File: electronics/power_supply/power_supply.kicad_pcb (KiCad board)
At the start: 2 copper layers, 7 parts, among them J1 INPUT, T1 RSPRO_121-3824, U1 NCP3334

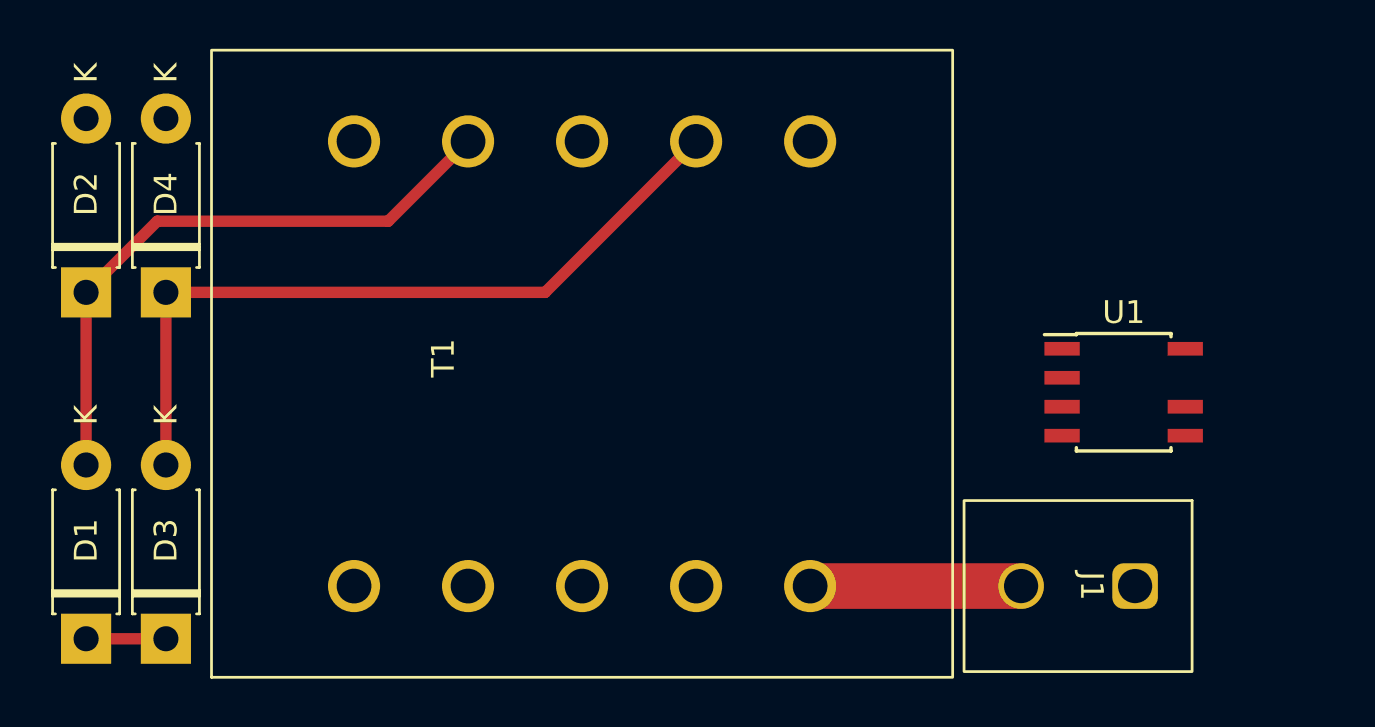
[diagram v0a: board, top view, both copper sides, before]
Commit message: power supply done, to check
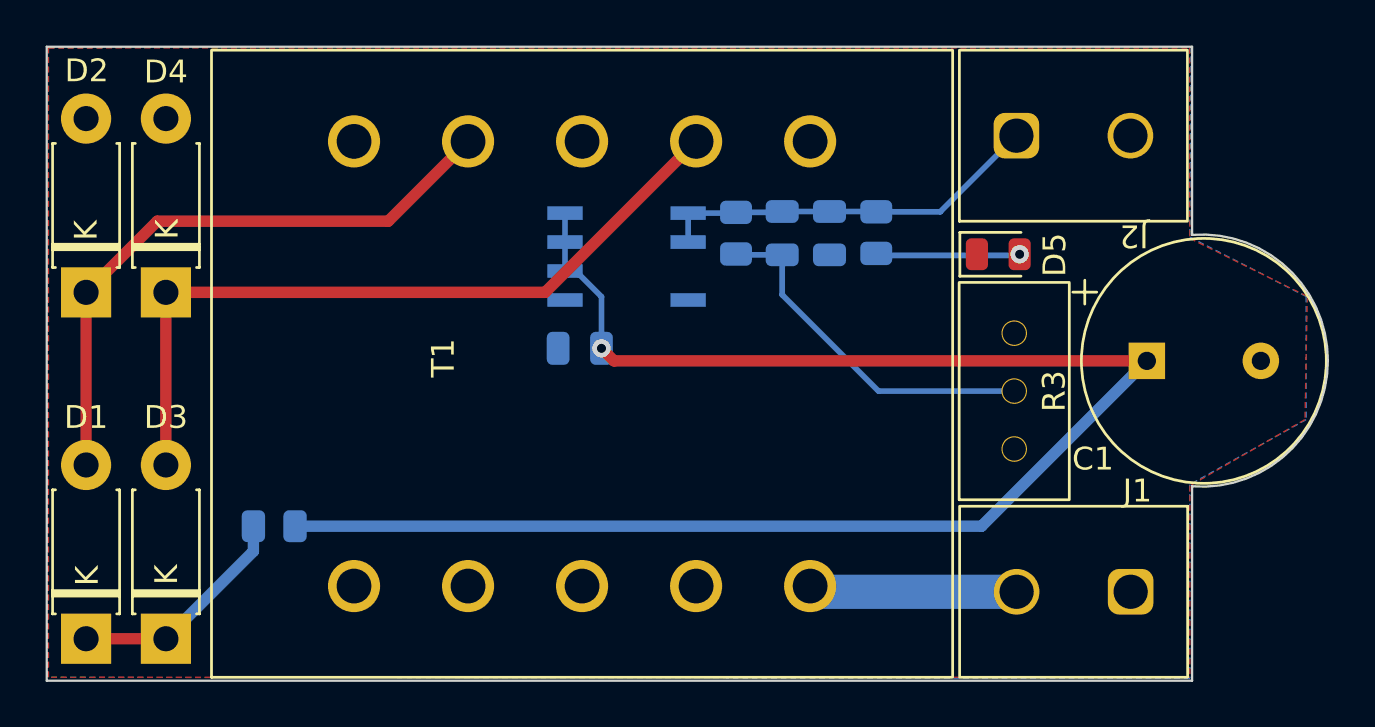
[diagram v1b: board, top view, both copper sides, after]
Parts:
- added C1: 470u, Capacitor_THT:CP_Radial_Tantal_D10.5mm_P5.00mm, F.Cu at (144.0, 56.6)
- added C2: 1u, Capacitor_SMD:C_0805_2012Metric, B.Cu at (119.2, 56.1)
- added C3: 68p, Capacitor_SMD:C_0805_2012Metric, B.Cu at (128.0, 51.0)
- added C4: 1u, Capacitor_SMD:C_0805_2012Metric, B.Cu at (130.1, 51.0)
- added D5: LED, Diode_SMD:D_0805_2012Metric, F.Cu at (137.5, 52.0)
- added J2: OUTPUT, USER:bornier_1x2_p5.00mm, F.Cu at (135.8, 46.8)
- added R1: 130, Resistor_SMD:R_0805_2012Metric, B.Cu at (105.8, 63.9)
- added R2: 1k, Resistor_SMD:R_0805_2012Metric, B.Cu at (126.0, 51.0)
- added R3: 100-1k, USER:3296W-1-102LF, F.Cu at (138.2, 58.0)
- added R4: 220, Resistor_SMD:R_0805_2012Metric, B.Cu at (132.2, 51.0)
- D1, D2, D3, D4: value DIODE -> 1N4007RLG
- U1: moved to B.Cu
- moved U1 22.6 mm to (121.2, 52.0)
- moved J1 0.32 mm to (145.8, 66.8)
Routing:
- net REGIN: track 0.00 -> 72.0 mm, vias 0 -> 1
- net REGOUT: track 0.00 -> 17.1 mm
- net Net-(C3-Pad2): track 0.00 -> 15.7 mm
- net VIN: track 3.50 -> 10.0 mm
- net Net-(D5-Pad2): track 0.00 -> 6.44 mm, vias 0 -> 1
- added copper zone on B.Cu, net NEUTRE
- added copper zone on F.Cu, net NEUTRE
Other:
- board outline added: 56.2 x 27.8 mm
